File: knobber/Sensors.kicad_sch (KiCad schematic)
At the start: 6 parts, among them U401 MT6701CT, U402 VEML7700-TT

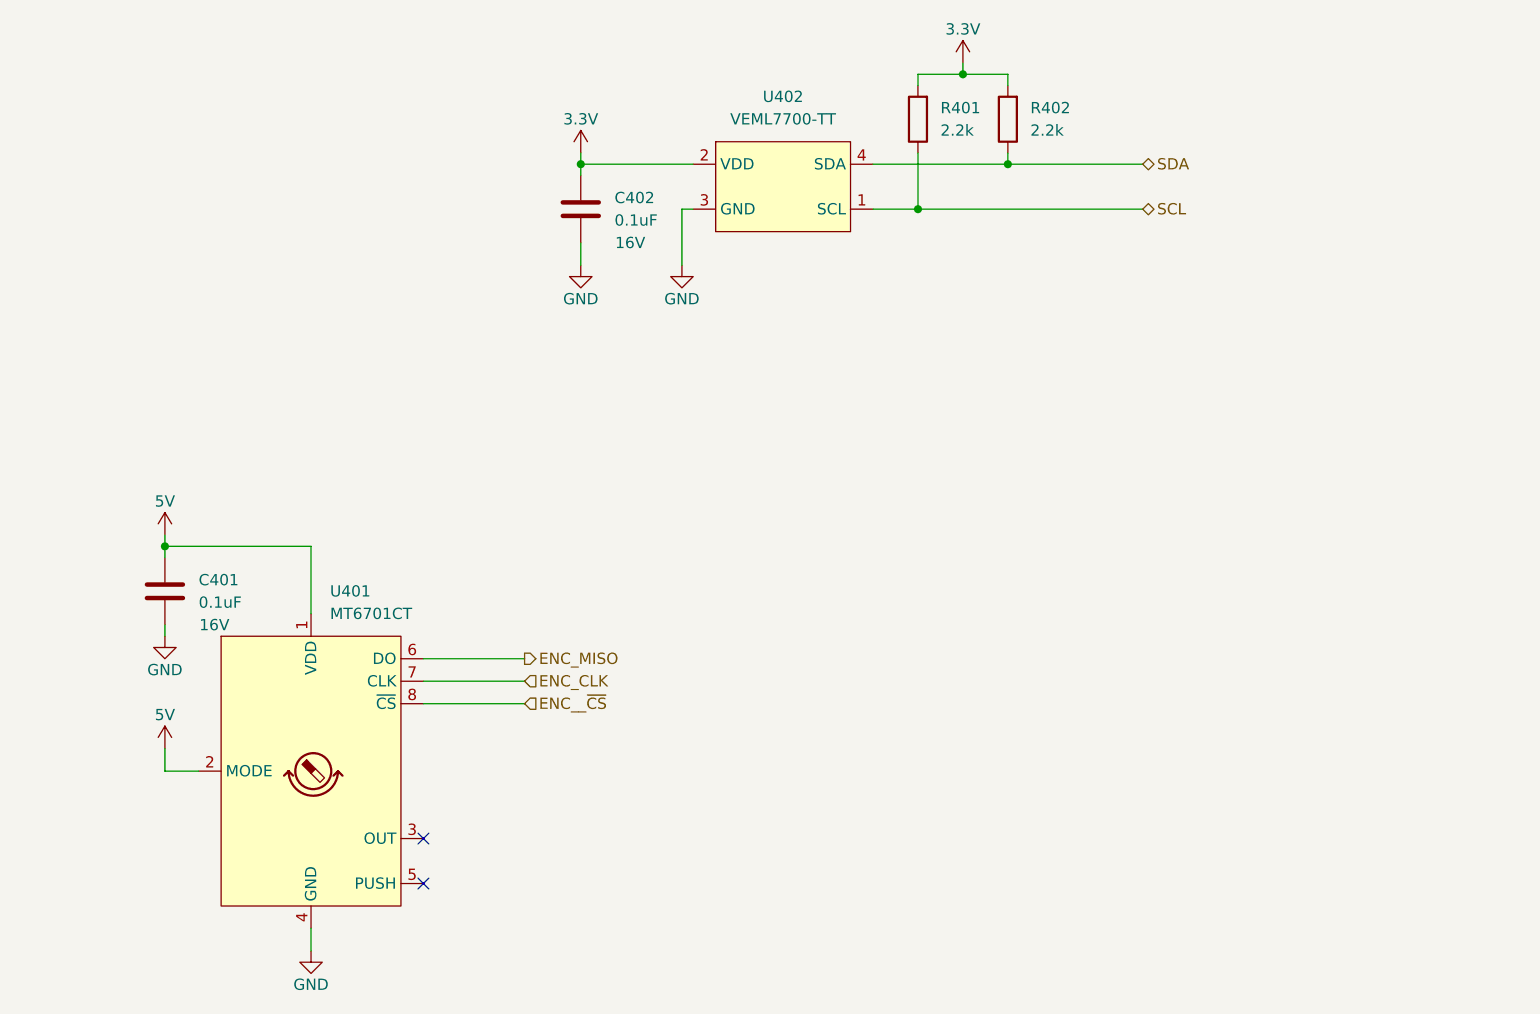
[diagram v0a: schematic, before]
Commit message: Updated schematic & PCB
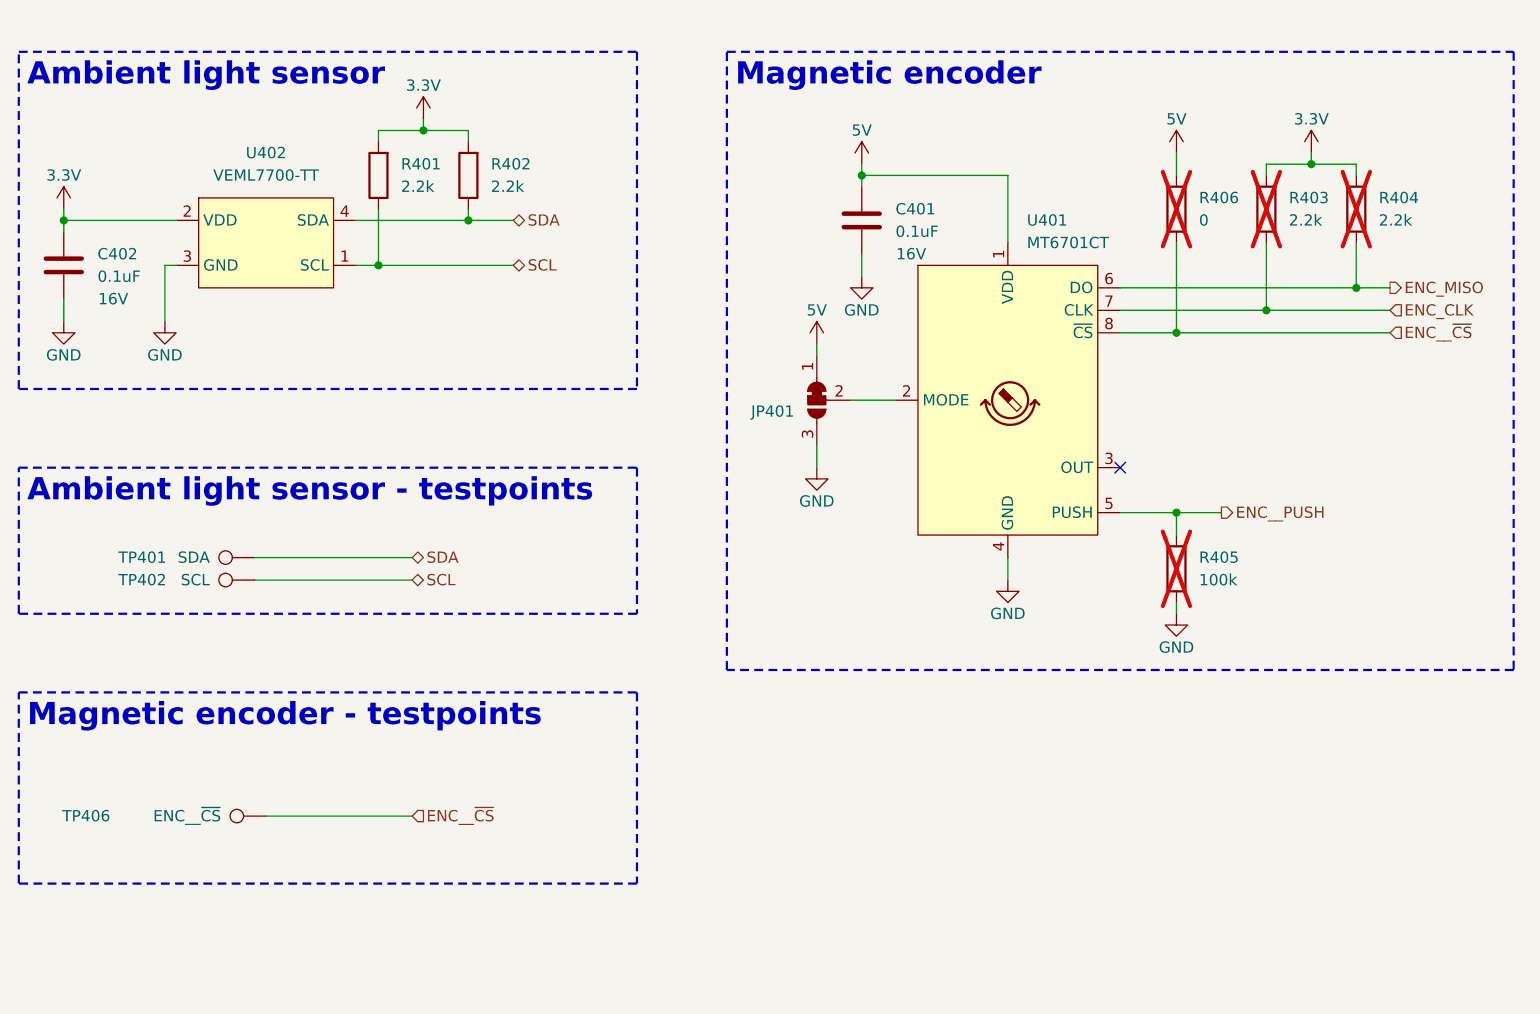
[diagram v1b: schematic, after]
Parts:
- added JP401: SolderJumper_3_Bridged12, Jumper:SolderJumper-3_P1.3mm_Bridged12_Pad1.0x1.5mm, symbol Jumper:SolderJumper_3_Bridged12
- added R403, R404: 2.2k, Resistor_SMD:R_0603_1608Metric, symbol Device:R
- added R405: 100k, Resistor_SMD:R_0603_1608Metric, symbol Device:R
- added R406: 0, Resistor_SMD:R_0603_1608Metric, symbol Device:R
- added TP401: SDA, TestPoint:TestPoint_Pad_D1.0mm, symbol Connector:TestPoint
- added TP402: SCL, TestPoint:TestPoint_Pad_D1.0mm, symbol Connector:TestPoint
- added TP406: ENC__~{CS}, TestPoint:TestPoint_Pad_D1.0mm, symbol Connector:TestPoint
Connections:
- net 3.3V: now also R403.2, R404.2
- net 5V: now also JP401.1 (A), R406.2; no longer U401.2 (MODE)
- net ENC_CLK: now also R403.1
- net ENC_MISO: now also R404.1
- net ENC__~{CS}: now also R406.1, TP406.1
- net GND: now also JP401.3 (B), R405.1
- net SCL: now also TP402.1
- net SDA: now also TP401.1
- net ENC__PUSH: now reaches U401.5 (PUSH)
- net ENC__PUSH: now also R405.2
- new net: JP401.2 (C), U401.2 (MODE)
- no-connect marks 2 -> 1
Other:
- moved on the sheet: C401, C402, R401, R402, U401, U402
